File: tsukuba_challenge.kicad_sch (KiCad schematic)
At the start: 26 parts, among them J1 PWR_BATT, J10 CAN, J2 USB_C_Receptacle_USB2.0, J3 ST-LINK, J4 INDICATOR, J5 INDICATOR, J6 INDICATOR, J7 CAN, J8 CAN, J9 CAN, Q1 TBD62083AFWG_Z,EHZ, U1 USBLC6-2SC6

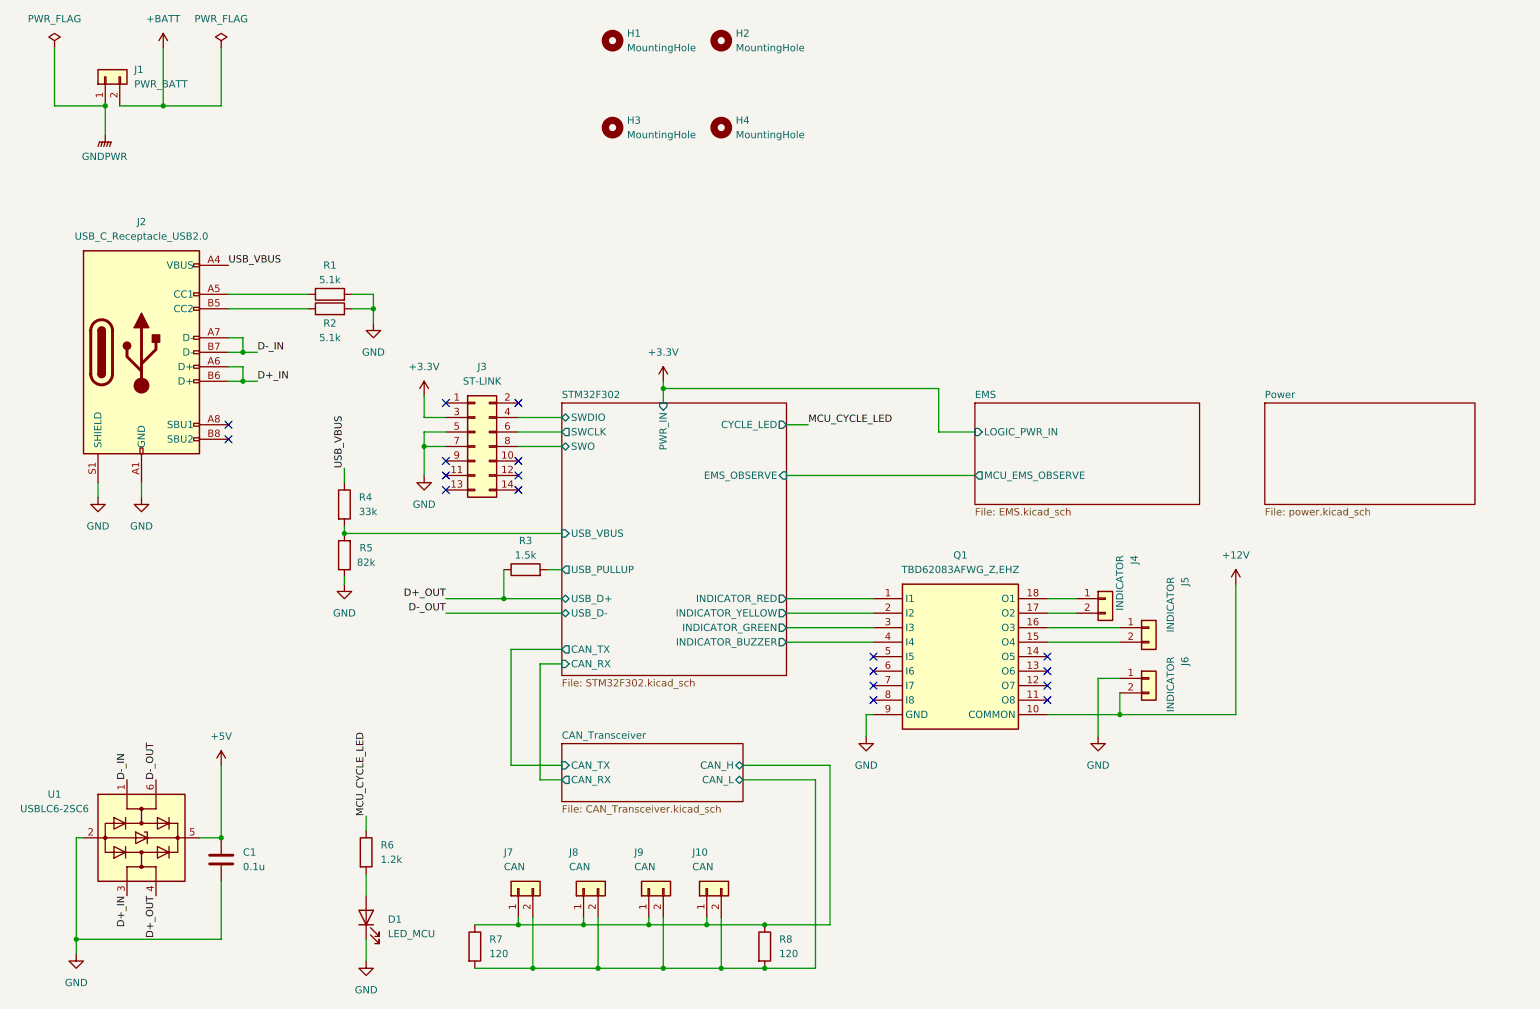
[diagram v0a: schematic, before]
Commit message: 5/28 kicad sch
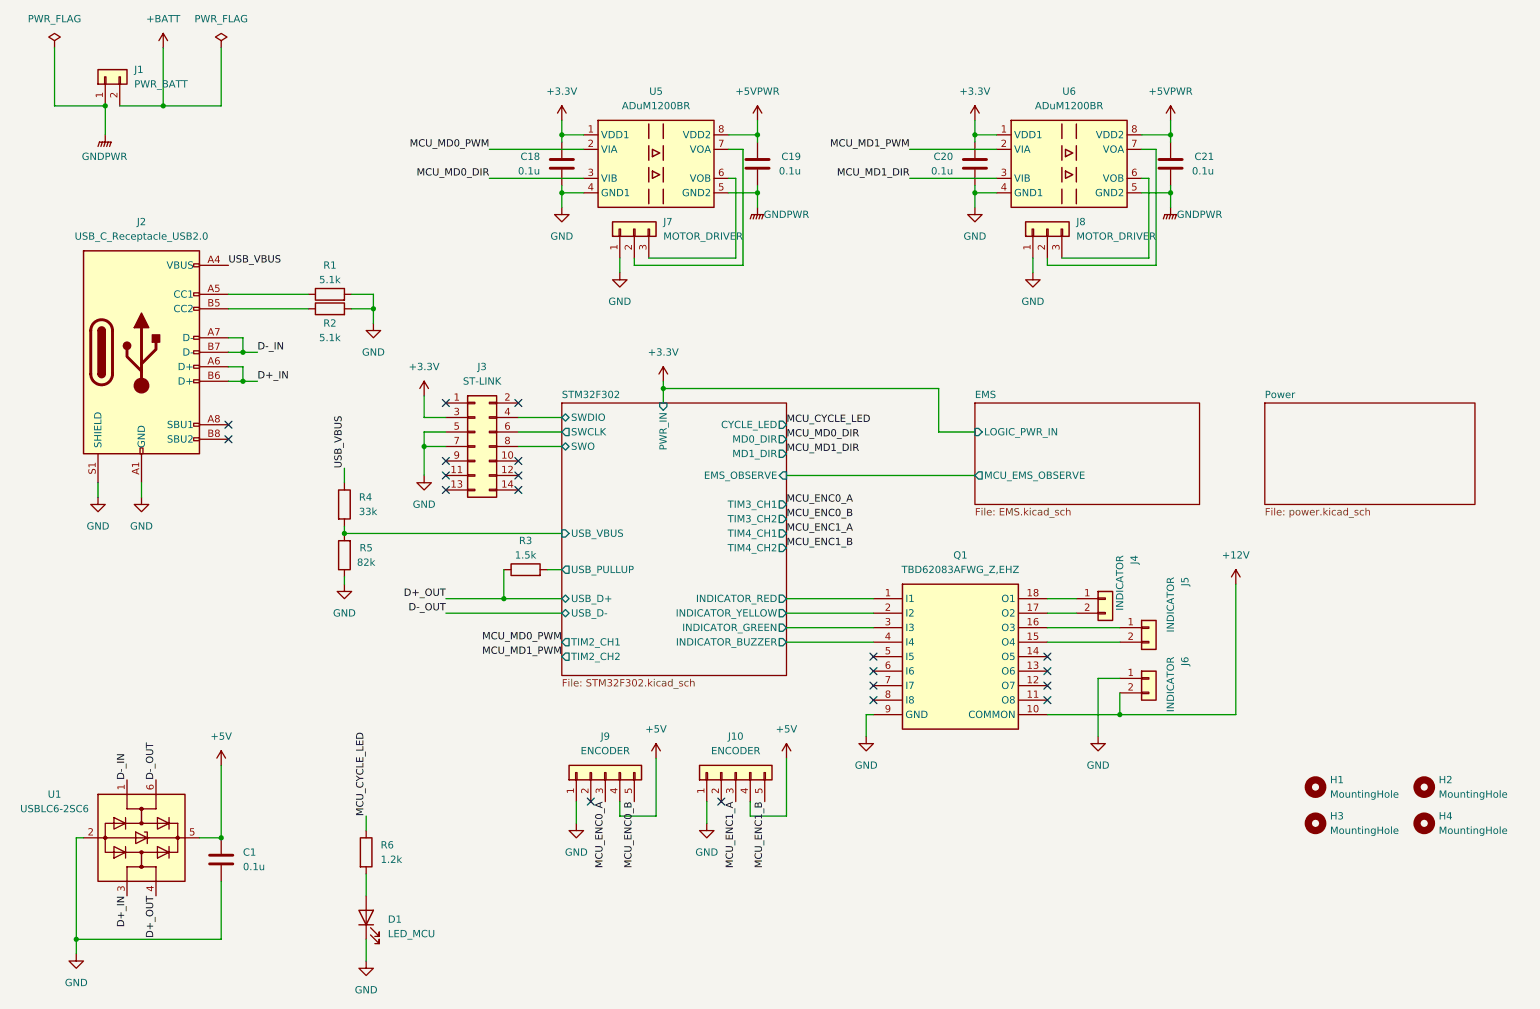
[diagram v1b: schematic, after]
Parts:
- removed J10, J7, J8, J9: CAN, Connector_JST:JST_XA_B02B-XASK-1_1x02_P2.50mm_Vertical, symbol Connector_Generic:Conn_01x02
- removed R7, R8: 120, Resistor_SMD:R_0603_1608Metric, symbol Device:R
- added C18, C19, C20, C21: 0.1u, Capacitor_SMD:C_0603_1608Metric, symbol Device:C
- added J10, J9: ENCODER, symbol Connector_Generic:Conn_01x05
- added J7, J8: MOTOR_DRIVER, symbol Connector_Generic:Conn_01x03
- added U5, U6: ADuM1200BR, Package_SO:SOIC-8_3.9x4.9mm_P1.27mm, symbol Isolator:ADuM1200BR
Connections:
- net +3.3V: now also C18.2, C20.2, U5.1 (VDD1), U6.1 (VDD1)
- net +5V: now also J10.4 (Pin_4), J9.4 (Pin_4)
- net GND: now also C18.1, C20.1, J10.1 (Pin_1), J7.1 (Pin_1), J8.1 (Pin_1), J9.1 (Pin_1), U5.4 (GND1), U6.4 (GND1)
- net GNDPWR: now also C19.1, C21.1, U5.5 (GND2), U6.5 (GND2)
- new net: J7.3 (Pin_3), U5.6 (VOB)
- new net: J7.2 (Pin_2), U5.7 (VOA)
- new net: J8.3 (Pin_3), U6.6 (VOB)
- new net: J8.2 (Pin_2), U6.7 (VOA)
- new net +5VPWR: C19.2, C21.2, U5.8 (VDD2), U6.8 (VDD2)
- new net MCU_ENC0_A: J9.3 (Pin_3)
- new net MCU_ENC0_B: J9.5 (Pin_5)
- new net MCU_ENC1_A: J10.3 (Pin_3)
- new net MCU_ENC1_B: J10.5 (Pin_5)
- new net MCU_MD0_DIR: U5.3 (VIB)
- new net MCU_MD0_PWM: U5.2 (VIA)
- new net MCU_MD1_DIR: U6.3 (VIB)
- new net MCU_MD1_PWM: U6.2 (VIA)
- no-connect marks 18 -> 20
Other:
- removed sheet CAN_Transceiver
- sheet STM32F302 ports: added MD0_DIR, MD1_DIR, TIM2_CH1, TIM2_CH2, TIM3_CH1, TIM3_CH2, TIM4_CH1, TIM4_CH2; removed CAN_RX, CAN_TX
- moved on the sheet: H1, H2, H3, H4
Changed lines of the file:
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@@
-(kicad_sch (version 20230121) (generator eeschema)
-  (paper "A4")
+(kicad_sch
+	(version 20260306)
+	(generator "eeschema")
+	(generator_version "10.0")
+	(paper "A4")
